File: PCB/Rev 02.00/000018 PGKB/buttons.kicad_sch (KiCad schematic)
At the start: 39 parts, among them U1 SN74HCS365PWR, U2 SN74HCS365PWR

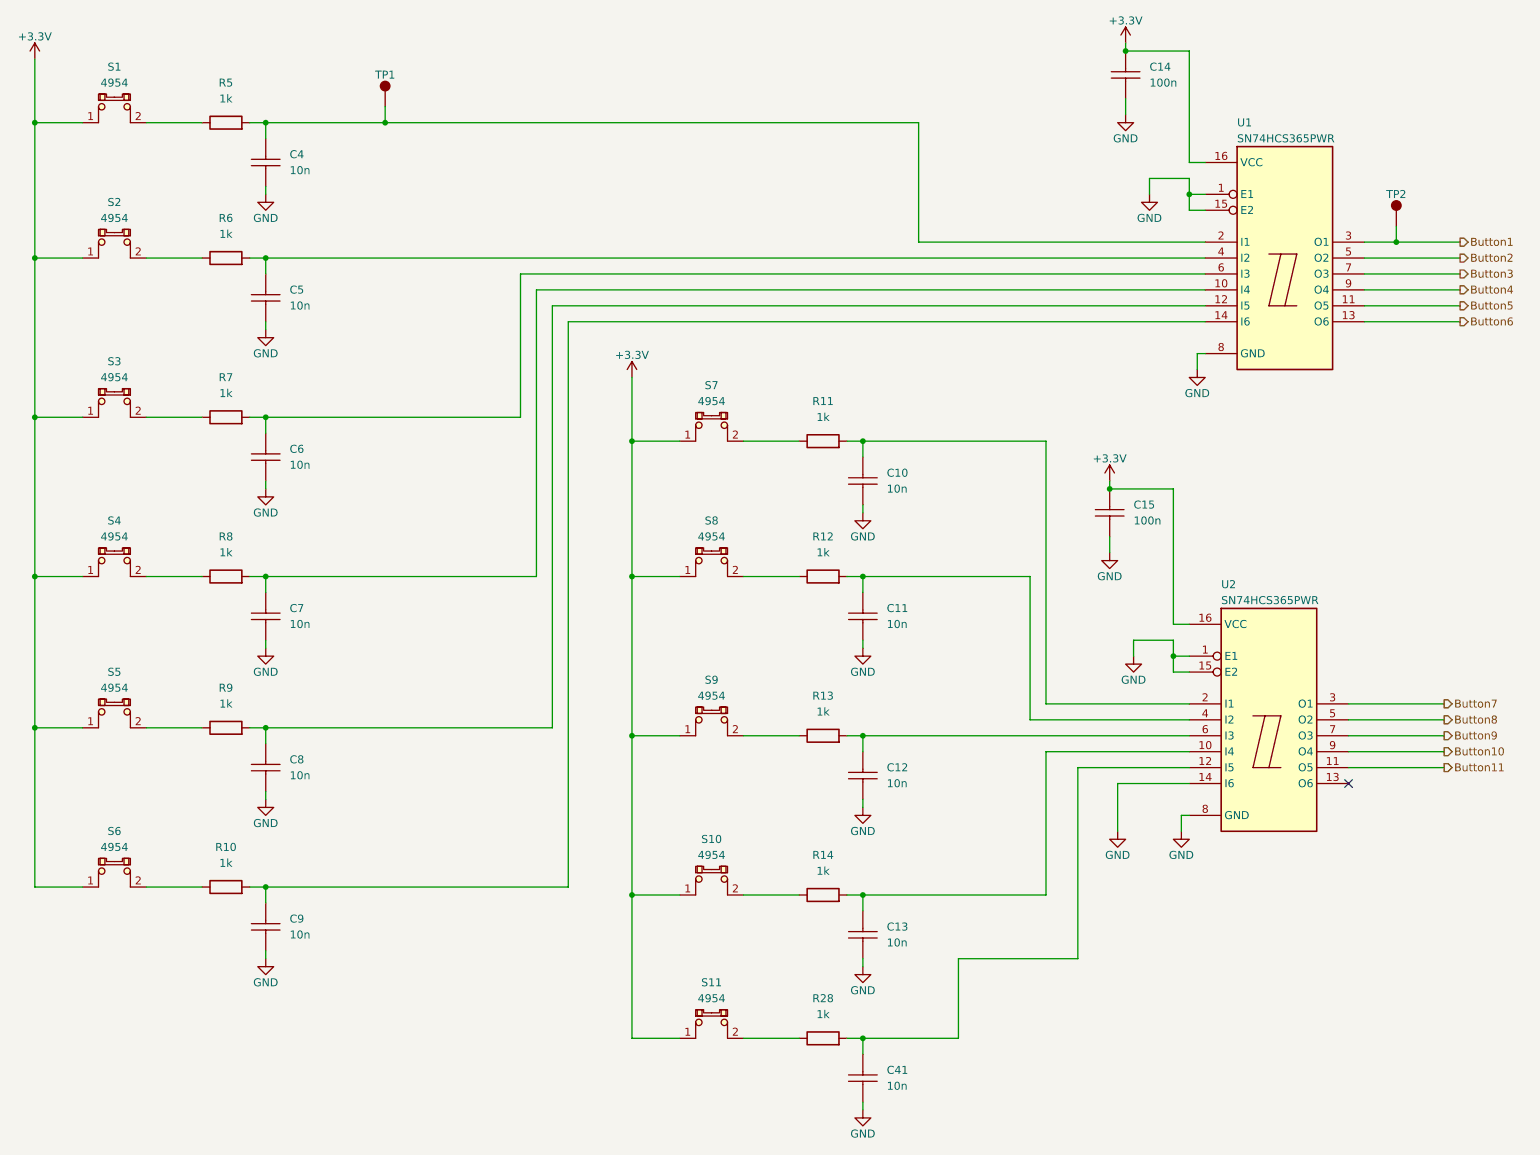
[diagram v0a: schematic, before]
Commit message: sitte vaan routaus
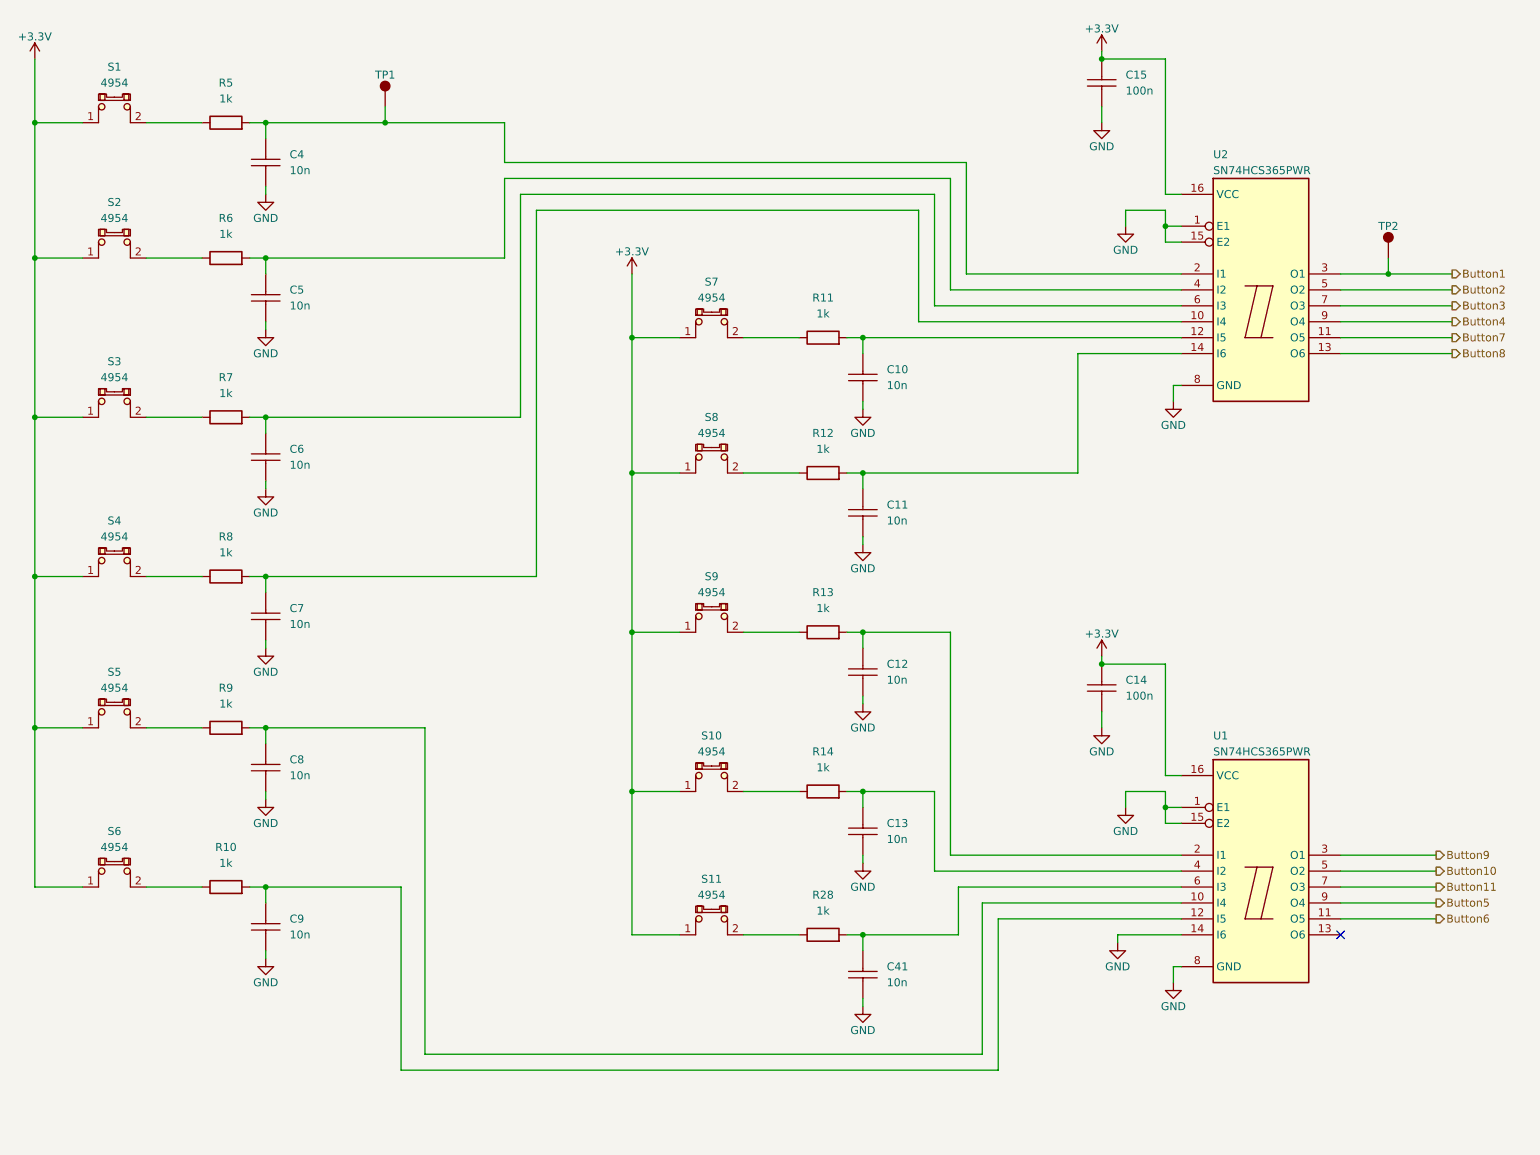
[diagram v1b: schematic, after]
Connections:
- net Button1: now also U2.3 (O1); no longer U1.3 (O1)
- net Button10: now also U1.5 (O2); no longer U2.9 (O4)
- net Button11: now also U1.7 (O3); no longer U2.11 (O5)
- net Button2: now also U2.5 (O2); no longer U1.5 (O2)
- net Button3: now also U2.7 (O3); no longer U1.7 (O3)
- net Button4: now also U2.9 (O4); no longer U1.9 (O4)
- net Button5: now also U1.9 (O4); no longer U1.11 (O5)
- net Button6: now also U1.11 (O5); no longer U1.13 (O6)
- net Button7: now also U2.11 (O5); no longer U2.3 (O1)
- net Button8: now also U2.13 (O6); no longer U2.5 (O2)
- net Button9: now also U1.3 (O1); no longer U2.7 (O3)
- net GND: now also U1.14 (I6); no longer U2.14 (I6)
- net at C7.1, R8.2: now also U2.10 (I4); no longer U1.10 (I4)
- net at C41.1, R28.2: now also U1.6 (I3); no longer U2.12 (I5)
- net at C13.1, R14.2: now also U1.4 (I2); no longer U2.10 (I4)
- net at C6.1, R7.2: now also U2.6 (I3); no longer U1.6 (I3)
- net at C8.1, R9.2: now also U1.10 (I4); no longer U1.12 (I5)
- net at C4.1, R5.2, TP1.1: now also U2.2 (I1); no longer U1.2 (I1)
- net at C9.1, R10.2: now also U1.12 (I5); no longer U1.14 (I6)
- net at C5.1, R6.2: now also U2.4 (I2); no longer U1.4 (I2)
- net at C10.1, R11.2: now also U2.12 (I5); no longer U2.2 (I1)
- net at C11.1, R12.2: now also U2.14 (I6); no longer U2.4 (I2)
- net at C12.1, R13.2: now also U1.2 (I1); no longer U2.6 (I3)
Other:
- moved on the sheet: C10, C11, C12, C13, C14, C15, C41, R11, R12, R13, R14, R28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
